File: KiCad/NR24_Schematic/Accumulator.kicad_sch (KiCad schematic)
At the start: 7 parts, among them K1 Relay, K3 Relay, K4 Relay, U8 Orian Jr 2 BMS

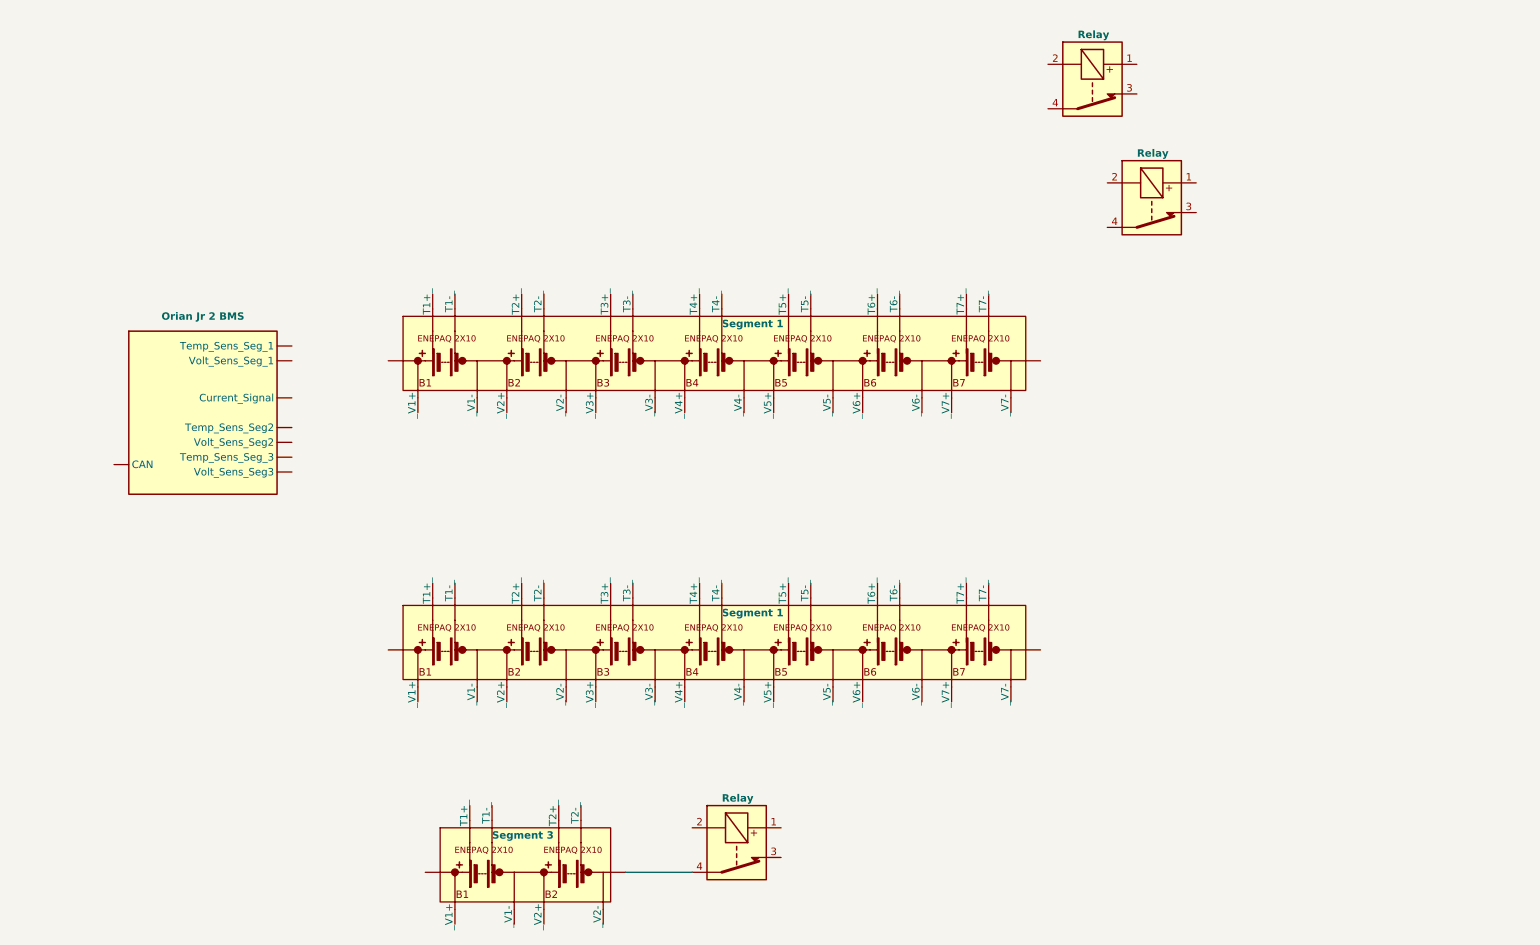
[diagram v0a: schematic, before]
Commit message: more stuff
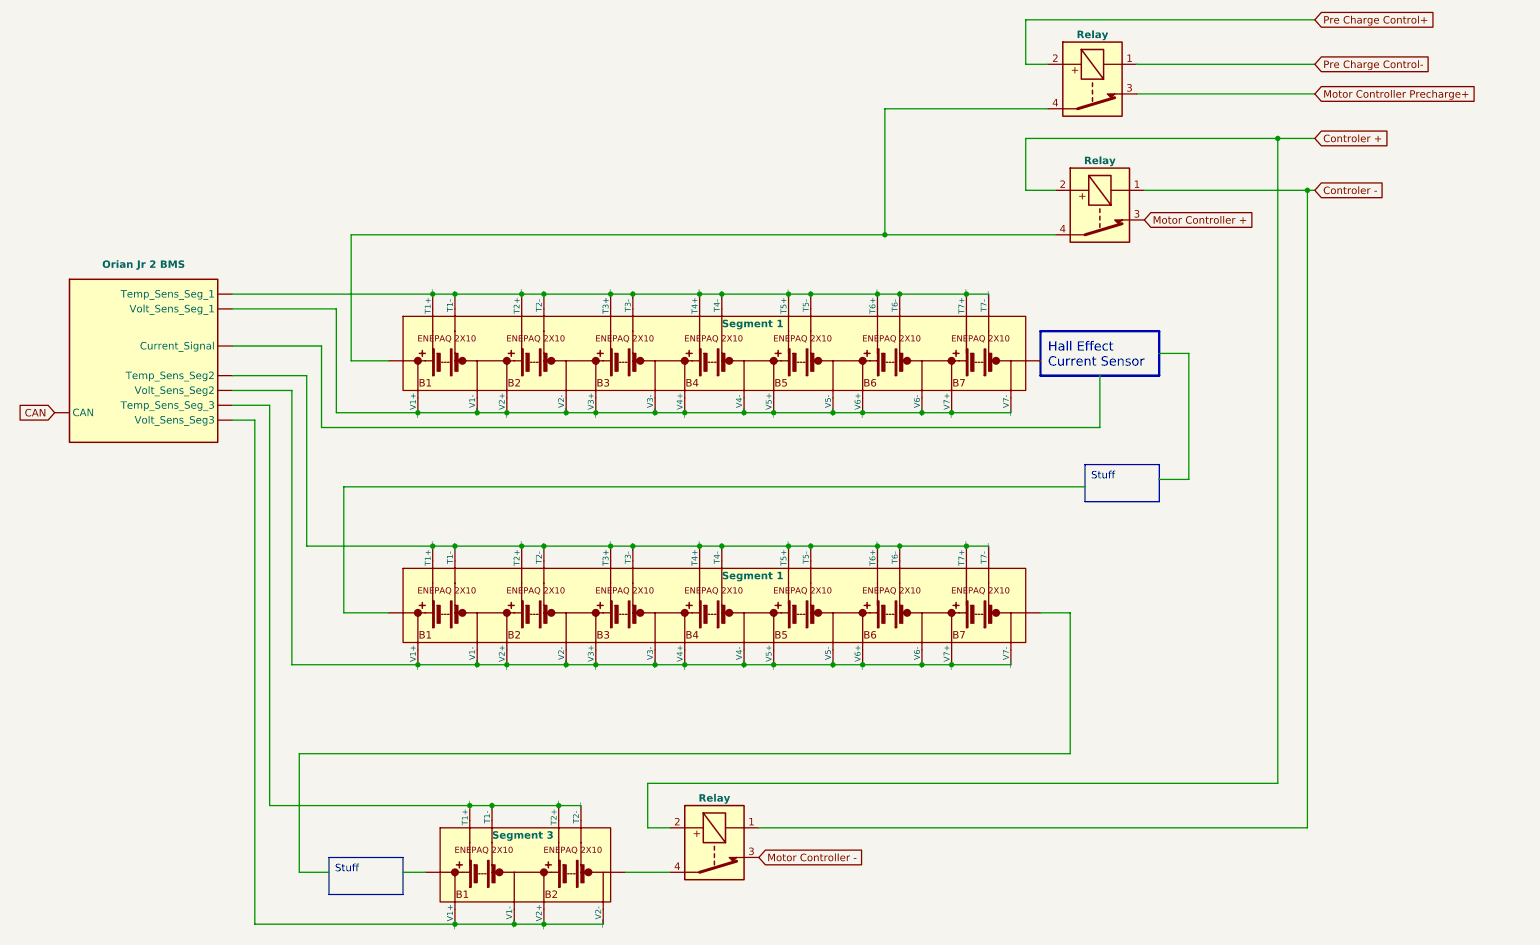
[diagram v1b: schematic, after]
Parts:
- removed BT5: Segment 1, symbol Device:Battery
- added BT3: Segment 1, symbol Device:Battery
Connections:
- net Controler -: now reaches K1.1
- net Controler -: now also K4.1
- net Controler +: now reaches K1.2
- net Controler +: now also K4.2
- net Motor Controller -: now reaches K1.3
- net CAN: now reaches U8. (Volt_Sens_Seg_1)
- net Motor Controller +: now reaches K4.3
- net at K4.4: now also BT2. (__V7-), K3.4
- net Pre Charge Control-: now reaches K3.1
- net Pre Charge Control+: now reaches K3.2
- net Motor Controller Precharge+: now reaches K3.3
- net at BT6.1 (T2+__): now also BT6.2 (T2-__), U8. (Volt_Sens_Seg_1)
- net at BT2.1 (T7+__): now also BT2.2 (T7-__), U8. (Volt_Sens_Seg_1)
- new net: BT6. (__V2-), U8. (Volt_Sens_Seg_1)
- new net: BT3. (__V7-), U8. (Volt_Sens_Seg_1)
- new net: BT3.1 (T7+__), BT3.2 (T7-__), U8. (Volt_Sens_Seg_1)
- new net: BT2. (__V7-), U8. (Volt_Sens_Seg_1)
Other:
- note added: "Hall Effect Current Sensor"

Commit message: first iteration
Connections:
- net at BT6. (__V2-): now also K1.4; no longer U8. (Volt_Sens_Seg_1)
- net at BT3. (__V7-): no longer U8. (Volt_Sens_Seg_1)
- net at BT2. (__V7-): no longer U8. (Volt_Sens_Seg_1)
- new net: BT6. (__V2-), U8. (Volt_Sens_Seg_1)
- new net: BT3. (__V7-), U8. (Volt_Sens_Seg_1)
- new net: BT2. (__V7-), U8. (Volt_Sens_Seg_1)

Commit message: Pre Break Schematic
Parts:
- renumbered BT2 to BT3, BT3 to BT4, BT6 to BT5, K3 to K2, K4 to K3, K1 to K4, U8 to U9
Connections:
- net at BT5. (__V2-): now also K4.4; no longer U9. (Volt_Sens_Seg_1)
- net at BT4. (__V7-): no longer U9. (Volt_Sens_Seg_1)
- net at BT3. (__V7-): no longer U9. (Volt_Sens_Seg_1)
- new net: BT5. (__V2-), U9. (Volt_Sens_Seg_1)
- new net: BT4. (__V7-), U9. (Volt_Sens_Seg_1)
- new net: BT3. (__V7-), U9. (Volt_Sens_Seg_1)
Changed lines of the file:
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@@
   (symbol (lib_name "EE2-4.5NU_1") (lib_id "Relay:EE2-4.5NU") (at 209.55 53.34 0) (unit 1)
     (in_bom yes) (on_board yes) (dnp no)
-    (property "Reference" "K4" (at 208.28 41.91 0)
+    (property "Reference" "K3" (at 208.28 41.91 0)
       (effects (font (size 1.27 1.27)) (justify left) hide)
     )
@@
     (pin "4")
     (instances
-      (project "Car_TractiveSystem_MAIN"
-        (path "/588b5c14-1813-4e1d-9dbe-940839ecebe3/600c7e11-1cec-4d55-8384-7f41b96b4c2b/6786b777-9654-4b97-bafc-3834bef66455"
-          (reference "K4") (unit 1)
+      (project "NR24_Schematic"
+        (path "/588b5c14-1813-4e1d-9dbe-940839ecebe3/600c7e11-1cec-4d55-8384-7f41b96b4c2b/6786b777-9654-4b97-bafc-3834bef66455"
+          (reference "K3") (unit 1)
         )
       )
@@
   (symbol (lib_id "Battery_Management:ADP5063") (at 45.72 77.47 0) (unit 1)
     (in_bom yes) (on_board yes) (dnp no) (fields_autoplaced)
-    (property "Reference" "U8" (at 45.72 59.69 0)
+    (property "Reference" "U9" (at 45.72 59.69 0)
       (effects (font (size 1.27 1.27)) hide)
     )
@@
     (pin "5")
     (instances
-      (project "Car_TractiveSystem_MAIN"
-        (path "/588b5c14-1813-4e1d-9dbe-940839ecebe3/600c7e11-1cec-4d55-8384-7f41b96b4c2b/6786b777-9654-4b97-bafc-3834bef66455"
-          (reference "U8") (unit 1)
+      (project "NR24_Schematic"
+        (path "/588b5c14-1813-4e1d-9dbe-940839ecebe3/600c7e11-1cec-4d55-8384-7f41b96b4c2b/6786b777-9654-4b97-bafc-3834bef66455"
+          (reference "U9") (unit 1)
         )
       )
@@
   (symbol (lib_name "EE2-4.5NU_1") (lib_id "Relay:EE2-4.5NU") (at 208.28 31.75 0) (unit 1)
     (in_bom yes) (on_board yes) (dnp no)
-    (property "Reference" "K3" (at 207.01 20.32 0)
+    (property "Reference" "K2" (at 207.01 20.32 0)
       (effects (font (size 1.27 1.27)) (justify left) hide)
     )
@@
     (pin "4")
     (instances
-      (project "Car_TractiveSystem_MAIN"
-        (path "/588b5c14-1813-4e1d-9dbe-940839ecebe3/600c7e11-1cec-4d55-8384-7f41b96b4c2b/6786b777-9654-4b97-bafc-3834bef66455"
-          (reference "K3") (unit 1)
+      (project "NR24_Schematic"
+        (path "/588b5c14-1813-4e1d-9dbe-940839ecebe3/600c7e11-1cec-4d55-8384-7f41b96b4c2b/6786b777-9654-4b97-bafc-3834bef66455"
+          (reference "K2") (unit 1)
         )
       )
@@
   (symbol (lib_name "Battery_2") (lib_id "Device:Battery") (at 110.49 166.37 0) (unit 1)
     (in_bom yes) (on_board yes) (dnp no) (fields_autoplaced)
-    (property "Reference" "BT6" (at 109.22 172.72 0)
+    (property "Reference" "BT5" (at 109.22 172.72 0)
       (effects (font (size 1.27 1.27)) (justify left) hide)
     )
@@
     (pin "2")
     (instances
-      (project "Car_TractiveSystem_MAIN"
-        (path "/588b5c14-1813-4e1d-9dbe-940839ecebe3/600c7e11-1cec-4d55-8384-7f41b96b4c2b/6786b777-9654-4b97-bafc-3834bef66455"
-          (reference "BT6") (unit 1)
+      (project "NR24_Schematic"
+        (path "/588b5c14-1813-4e1d-9dbe-940839ecebe3/600c7e11-1cec-4d55-8384-7f41b96b4c2b/6786b777-9654-4b97-bafc-3834bef66455"
+          (reference "BT5") (unit 1)
         )
       )
@@
   (symbol (lib_name "Battery_3") (lib_id "Device:Battery") (at 132.08 135.89 0) (unit 1)
     (in_bom yes) (on_board yes) (dnp no) (fields_autoplaced)
-    (property "Reference" "BT3" (at 140.97 129.54 0)
+    (property "Reference" "BT4" (at 140.97 129.54 0)
       (effects (font (size 1.27 1.27)) (justify left) hide)
     )
@@
     (pin "2")
     (instances
-      (project "Car_TractiveSystem_MAIN"
-        (path "/588b5c14-1813-4e1d-9dbe-940839ecebe3/600c7e11-1cec-4d55-8384-7f41b96b4c2b/6786b777-9654-4b97-bafc-3834bef66455"
-          (reference "BT3") (unit 1)
+      (project "NR24_Schematic"
+        (path "/588b5c14-1813-4e1d-9dbe-940839ecebe3/600c7e11-1cec-4d55-8384-7f41b96b4c2b/6786b777-9654-4b97-bafc-3834bef66455"
+          (reference "BT4") (unit 1)
         )
       )
@@
   (symbol (lib_name "EE2-4.5NU_1") (lib_id "Relay:EE2-4.5NU") (at 143.51 162.56 0) (unit 1)
     (in_bom yes) (on_board yes) (dnp no)
-    (property "Reference" "K1" (at 142.24 151.13 0)
+    (property "Reference" "K4" (at 142.24 151.13 0)
       (effects (font (size 1.27 1.27)) (justify left) hide)
     )
@@
     (pin "4")
     (instances
-      (project "Car_TractiveSystem_MAIN"
-        (path "/588b5c14-1813-4e1d-9dbe-940839ecebe3/600c7e11-1cec-4d55-8384-7f41b96b4c2b/6786b777-9654-4b97-bafc-3834bef66455"
-          (reference "K1") (unit 1)
+      (project "NR24_Schematic"
+        (path "/588b5c14-1813-4e1d-9dbe-940839ecebe3/600c7e11-1cec-4d55-8384-7f41b96b4c2b/6786b777-9654-4b97-bafc-3834bef66455"
+          (reference "K4") (unit 1)
         )
       )
@@
   (symbol (lib_name "Battery_3") (lib_id "Device:Battery") (at 132.08 92.71 0) (unit 1)
     (in_bom yes) (on_board yes) (dnp no) (fields_autoplaced)
-    (property "Reference" "BT2" (at 140.97 86.36 0)
+    (property "Reference" "BT3" (at 140.97 86.36 0)
       (effects (font (size 1.27 1.27)) (justify left) hide)
     )
@@
     (pin "2")
     (instances
-      (project "Car_TractiveSystem_MAIN"
-        (path "/588b5c14-1813-4e1d-9dbe-940839ecebe3/600c7e11-1cec-4d55-8384-7f41b96b4c2b/6786b777-9654-4b97-bafc-3834bef66455"
-          (reference "BT2") (unit 1)
-        )
-      )
+      (project "NR24_Schematic"
+        (path "/588b5c14-1813-4e1d-9dbe-940839ecebe3/600c7e11-1cec-4d55-8384-7f41b96b4c2b/6786b777-9654-4b97-bafc-3834bef66455"
+          (reference "BT3") (unit 1)
+        )
+      )
